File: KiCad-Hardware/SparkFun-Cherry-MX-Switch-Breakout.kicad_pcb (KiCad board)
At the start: 2 copper layers, 19.1 x 19.1 mm, 16 parts

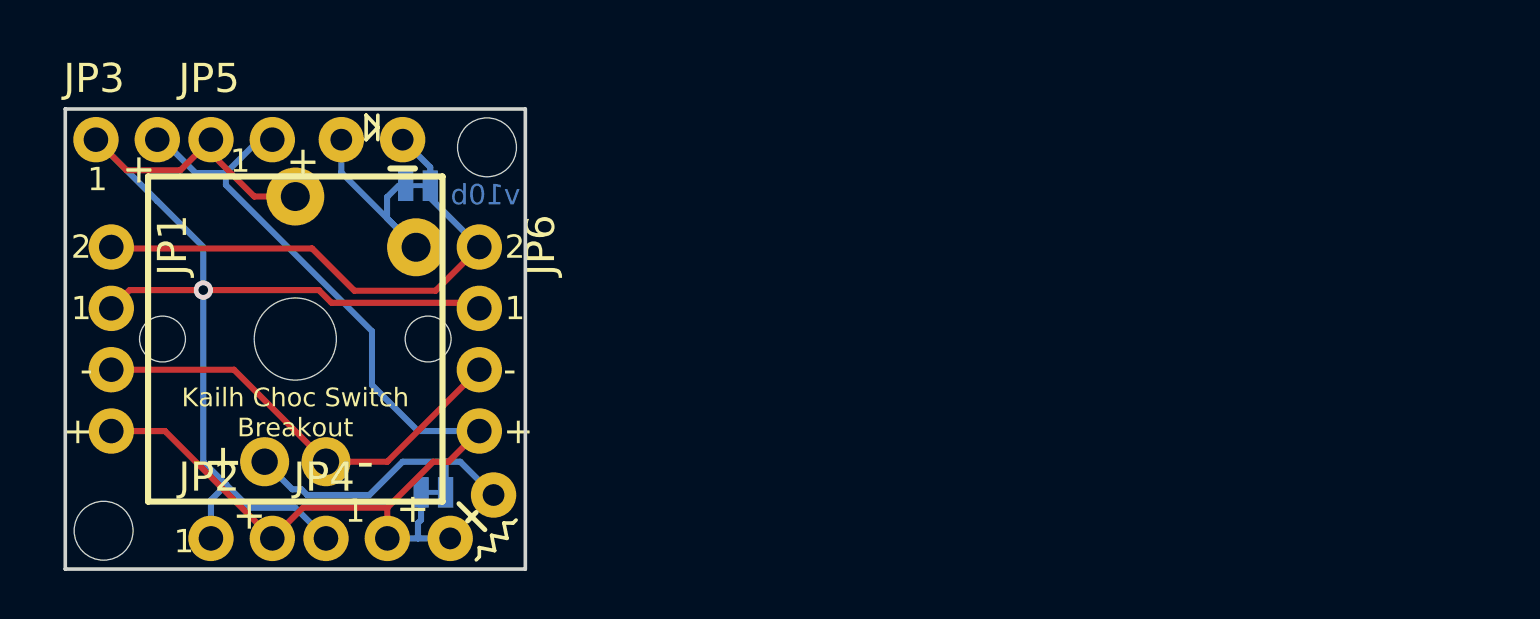
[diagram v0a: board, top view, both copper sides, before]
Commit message: Commit of triplet version
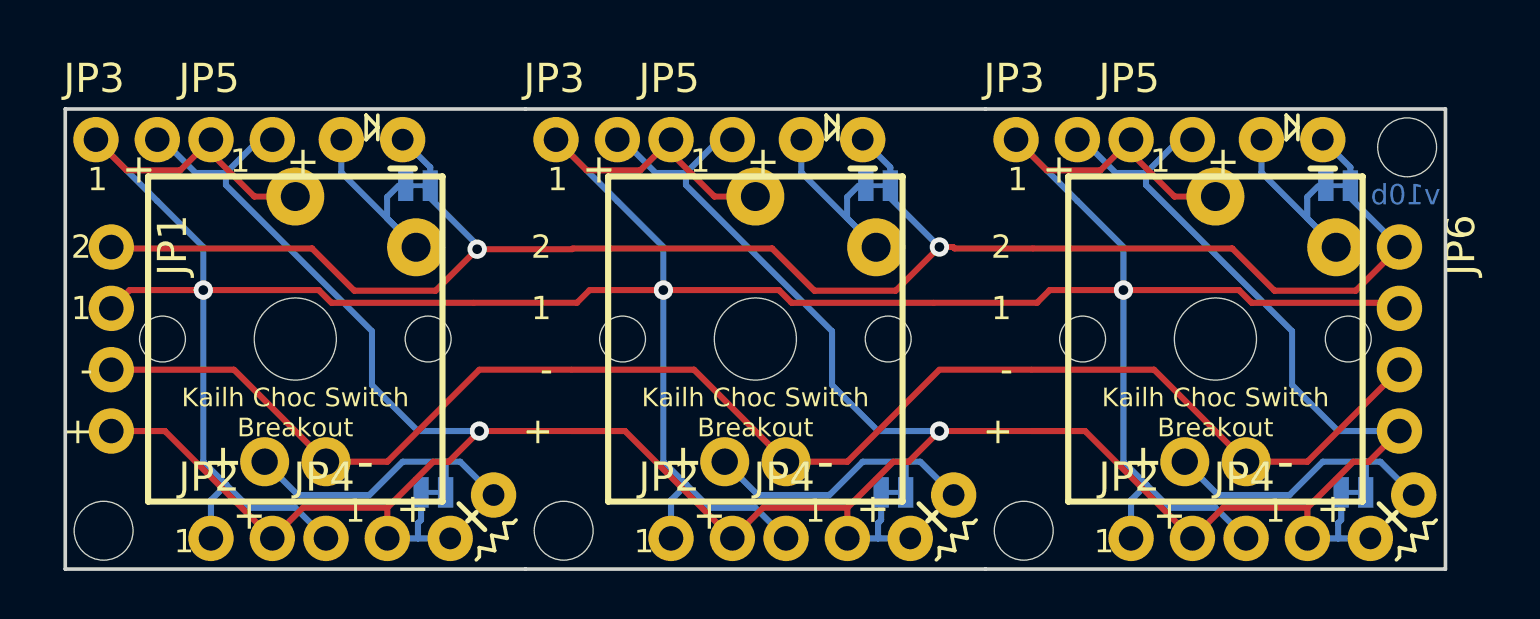
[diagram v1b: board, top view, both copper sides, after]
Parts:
- added D1: DNP, SparkFun-Cherry-MX-Switch-Breakout:DIODE-PTH-0.1, F.Cu at (191.3, 91.7)
- added D1: DNP, SparkFun-Cherry-MX-Switch-Breakout:DIODE-PTH-0.1, F.Cu at (172.2, 91.7)
- added JP2: M021X02_NO_SILK, SparkFun-Cherry-MX-Switch-Breakout:1X02_NO_SILK, F.Cu at (184.6, 108.3)
- added JP2: M021X02_NO_SILK, SparkFun-Cherry-MX-Switch-Breakout:1X02_NO_SILK, F.Cu at (165.6, 108.3)
- added JP3: M021X02_NO_SILK, SparkFun-Cherry-MX-Switch-Breakout:1X02_NO_SILK, F.Cu at (179.8, 91.7)
- added JP3: M021X02_NO_SILK, SparkFun-Cherry-MX-Switch-Breakout:1X02_NO_SILK, F.Cu at (160.8, 91.7)
- added JP4: M021X02_NO_SILK, SparkFun-Cherry-MX-Switch-Breakout:1X02_NO_SILK, F.Cu at (189.4, 108.3)
- added JP4: M021X02_NO_SILK, SparkFun-Cherry-MX-Switch-Breakout:1X02_NO_SILK, F.Cu at (170.3, 108.3)
- added JP5: M021X02_NO_SILK, SparkFun-Cherry-MX-Switch-Breakout:1X02_NO_SILK, F.Cu at (184.6, 91.7)
- added JP5: M021X02_NO_SILK, SparkFun-Cherry-MX-Switch-Breakout:1X02_NO_SILK, F.Cu at (165.6, 91.7)
- added LOGO1: OSHW-LOGOS, SparkFun-Cherry-MX-Switch-Breakout:OSHW-LOGO-S, B.Cu at (182.6, 106.3)
- added LOGO1: OSHW-LOGOS, SparkFun-Cherry-MX-Switch-Breakout:OSHW-LOGO-S, B.Cu at (163.5, 106.3)
- added LOGO2: SFE_LOGO_FLAME.1_INCH, SparkFun-Cherry-MX-Switch-Breakout:SFE_LOGO_FLAME_.1, B.Cu at (191.9, 99.9)
- added LOGO2: SFE_LOGO_FLAME.1_INCH, SparkFun-Cherry-MX-Switch-Breakout:SFE_LOGO_FLAME_.1, B.Cu at (172.9, 99.9)
- added R1: DNP, SparkFun-Cherry-MX-Switch-Breakout:AXIAL-0.1, F.Cu at (194.5, 108.3)
- added R1: DNP, SparkFun-Cherry-MX-Switch-Breakout:AXIAL-0.1, F.Cu at (175.5, 108.3)
- added S1: CHERRY-MX-LED, SparkFun-Cherry-MX-Switch-Breakout:CHERRY-MX-LED, F.Cu at (188.1, 100.0)
- added S1: CHERRY-MX-LED, SparkFun-Cherry-MX-Switch-Breakout:CHERRY-MX-LED, F.Cu at (169.1, 100.0)
- added SJ1: JUMPER-PAD-2-NC_BY_TRACENO_SILK, SparkFun-Cherry-MX-Switch-Breakout:PAD-JUMPER-2-NC_BY_TRACE_NO_SILK, B.Cu at (193.8, 106.3)
- added SJ1: JUMPER-PAD-2-NC_BY_TRACENO_SILK, SparkFun-Cherry-MX-Switch-Breakout:PAD-JUMPER-2-NC_BY_TRACE_NO_SILK, B.Cu at (174.8, 106.3)
- added SJ2: JUMPER-PAD-2-NC_BY_TRACENO_SILK, SparkFun-Cherry-MX-Switch-Breakout:PAD-JUMPER-2-NC_BY_TRACE_NO_SILK, B.Cu at (193.2, 93.7)
- added SJ2: JUMPER-PAD-2-NC_BY_TRACENO_SILK, SparkFun-Cherry-MX-Switch-Breakout:PAD-JUMPER-2-NC_BY_TRACE_NO_SILK, B.Cu at (174.1, 93.7)
- added STANDOFF2: STAND-OFF2-56, SparkFun-Cherry-MX-Switch-Breakout:STAND-OFF-2-56, F.Cu at (180.2, 107.9)
- added STANDOFF2: STAND-OFF2-56, SparkFun-Cherry-MX-Switch-Breakout:STAND-OFF-2-56, F.Cu at (161.1, 107.9)
- moved JP6 38.1 mm to (195.7, 96.2)
- moved STANDOFF1 38.1 mm to (196.0, 92.1)
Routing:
- net /SWITCH1: track 50.5 -> 158.8 mm, vias 1 -> 3
- net /LEDA: track 47.2 -> 149.2 mm, vias 0 -> 2
- net /SWITCH2: track 22.5 -> 75.2 mm, vias 0 -> 2
- net /LEDC: track 18.4 -> 62.8 mm
- net Net-(R1-PadP$2): track 12.5 -> 37.4 mm
- net Net-(D1-PadA): track 8.98 -> 26.9 mm
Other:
- board size 19.1 x 19.1 mm -> 57.2 x 19.1 mm
